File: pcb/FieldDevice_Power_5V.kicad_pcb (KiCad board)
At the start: 2 copper layers, 25 parts, among them J1 Itp_1, J2 V in 6-18V, J3 Itp_2, J4 V out 5V, J5 Vtp_2, J6 Vtp_1, J7 Battery, U1 TPS54232

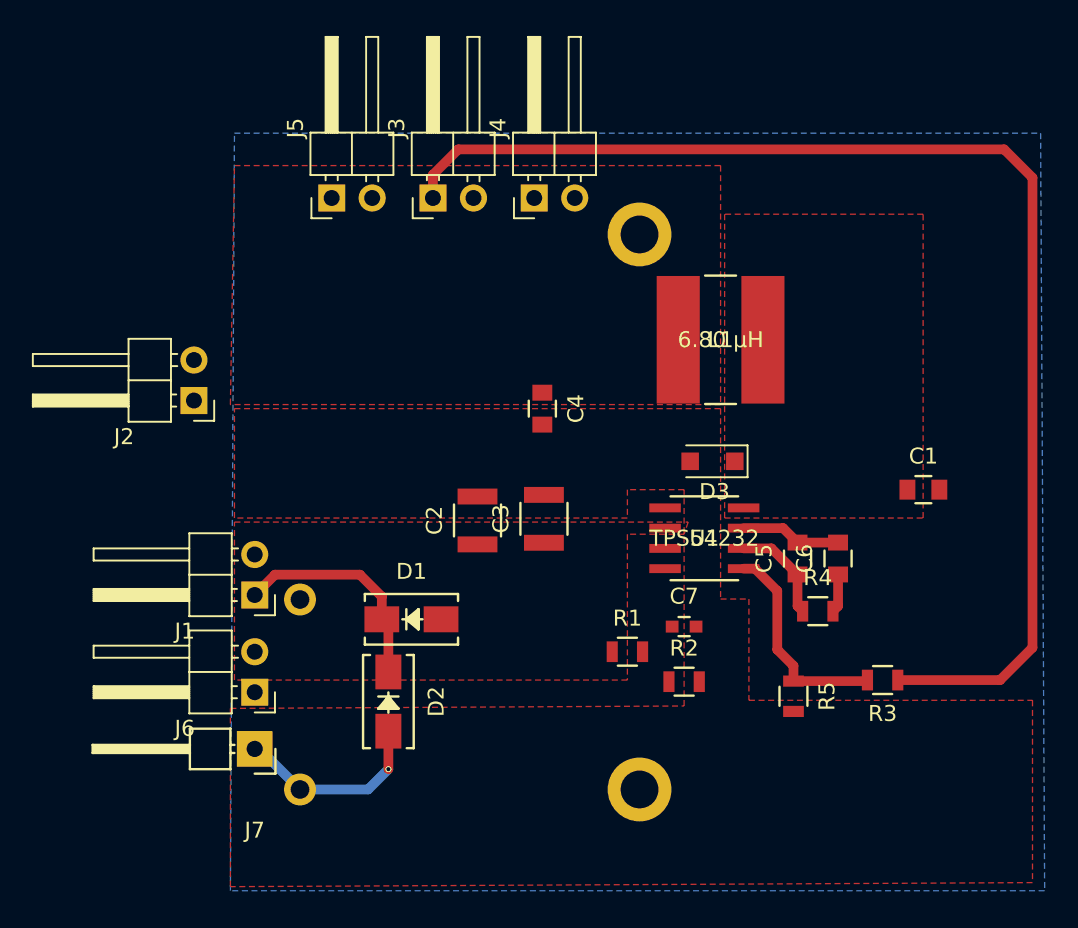
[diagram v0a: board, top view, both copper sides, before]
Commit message: Finishing up the layout
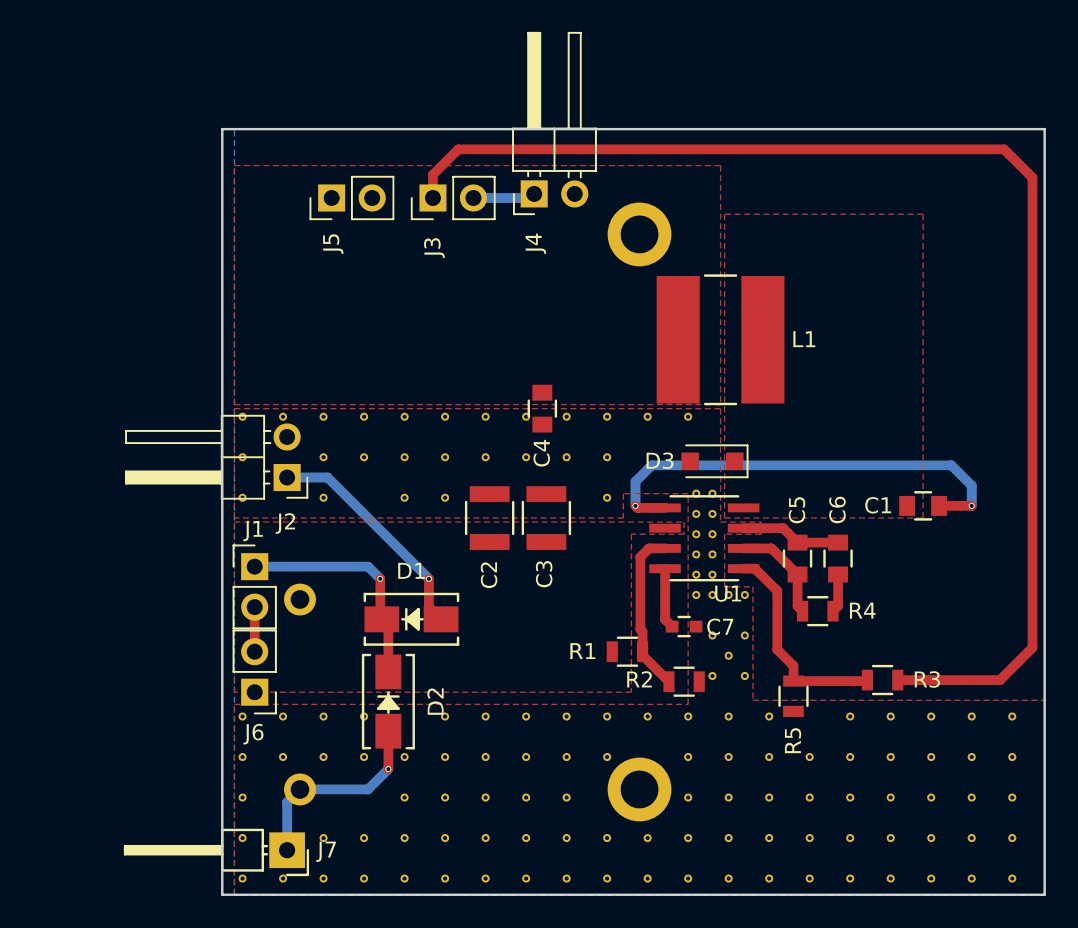
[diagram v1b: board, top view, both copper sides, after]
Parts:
- added ST**: STITCH_VIA, FieldDevice_Power_5V:STITCH_VIA, F.Cu at (95.8, 77.2)
- added ST**: STITCH_VIA, FieldDevice_Power_5V:STITCH_VIA, F.Cu at (94.7, 73.4)
- added ST**: STITCH_VIA, FieldDevice_Power_5V:STITCH_VIA, F.Cu at (93.2, 81.0)
- added ST**: STITCH_VIA, FieldDevice_Power_5V:STITCH_VIA, F.Cu at (90.7, 81.0)
- added ST**: STITCH_VIA, FieldDevice_Power_5V:STITCH_VIA, F.Cu at (88.1, 81.0)
- added ST**: STITCH_VIA, FieldDevice_Power_5V:STITCH_VIA, F.Cu at (85.6, 81.0)
- added ST**: STITCH_VIA, FieldDevice_Power_5V:STITCH_VIA, F.Cu at (83.1, 81.0)
- added ST**: STITCH_VIA, FieldDevice_Power_5V:STITCH_VIA, F.Cu at (80.5, 81.0)
- added ST**: STITCH_VIA, FieldDevice_Power_5V:STITCH_VIA, F.Cu at (78.0, 81.0)
- added ST**: STITCH_VIA, FieldDevice_Power_5V:STITCH_VIA, F.Cu at (72.9, 81.0)
- added ST**: STITCH_VIA, FieldDevice_Power_5V:STITCH_VIA, F.Cu at (70.4, 81.0)
- added ST**: STITCH_VIA, FieldDevice_Power_5V:STITCH_VIA, F.Cu at (67.8, 81.0)
- added ST**: STITCH_VIA, FieldDevice_Power_5V:STITCH_VIA, F.Cu at (94.7, 72.1)
- added ST**: STITCH_VIA, FieldDevice_Power_5V:STITCH_VIA, F.Cu at (65.3, 81.0)
- added ST**: STITCH_VIA, FieldDevice_Power_5V:STITCH_VIA, F.Cu at (88.1, 67.3)
- added ST**: STITCH_VIA, FieldDevice_Power_5V:STITCH_VIA, F.Cu at (78.0, 67.3)
- added ST**: STITCH_VIA, FieldDevice_Power_5V:STITCH_VIA, F.Cu at (75.4, 67.3)
- added ST**: STITCH_VIA, FieldDevice_Power_5V:STITCH_VIA, F.Cu at (70.4, 67.3)
- added ST**: STITCH_VIA, FieldDevice_Power_5V:STITCH_VIA, F.Cu at (65.3, 67.3)
- added ST**: STITCH_VIA, FieldDevice_Power_5V:STITCH_VIA, F.Cu at (88.1, 64.8)
- added ST**: STITCH_VIA, FieldDevice_Power_5V:STITCH_VIA, F.Cu at (85.6, 64.8)
- added ST**: STITCH_VIA, FieldDevice_Power_5V:STITCH_VIA, F.Cu at (83.1, 64.8)
- added ST**: STITCH_VIA, FieldDevice_Power_5V:STITCH_VIA, F.Cu at (80.5, 64.8)
- added ST**: STITCH_VIA, FieldDevice_Power_5V:STITCH_VIA, F.Cu at (94.7, 70.9)
- added ST**: STITCH_VIA, FieldDevice_Power_5V:STITCH_VIA, F.Cu at (78.0, 64.8)
- added ST**: STITCH_VIA, FieldDevice_Power_5V:STITCH_VIA, F.Cu at (75.4, 64.8)
- added ST**: STITCH_VIA, FieldDevice_Power_5V:STITCH_VIA, F.Cu at (72.9, 64.8)
- added ST**: STITCH_VIA, FieldDevice_Power_5V:STITCH_VIA, F.Cu at (70.4, 64.8)
- added ST**: STITCH_VIA, FieldDevice_Power_5V:STITCH_VIA, F.Cu at (65.3, 64.8)
- added ST**: STITCH_VIA, FieldDevice_Power_5V:STITCH_VIA, F.Cu at (93.2, 62.2)
- added ST**: STITCH_VIA, FieldDevice_Power_5V:STITCH_VIA, F.Cu at (90.7, 62.2)
- added ST**: STITCH_VIA, FieldDevice_Power_5V:STITCH_VIA, F.Cu at (88.1, 62.2)
- added ST**: STITCH_VIA, FieldDevice_Power_5V:STITCH_VIA, F.Cu at (85.6, 62.2)
- added ST**: STITCH_VIA, FieldDevice_Power_5V:STITCH_VIA, F.Cu at (83.1, 62.2)
- added ST**: STITCH_VIA, FieldDevice_Power_5V:STITCH_VIA, F.Cu at (94.7, 69.6)
- added ST**: STITCH_VIA, FieldDevice_Power_5V:STITCH_VIA, F.Cu at (80.5, 62.2)
- added ST**: STITCH_VIA, FieldDevice_Power_5V:STITCH_VIA, F.Cu at (78.0, 62.2)
- added ST**: STITCH_VIA, FieldDevice_Power_5V:STITCH_VIA, F.Cu at (75.4, 62.2)
- added ST**: STITCH_VIA, FieldDevice_Power_5V:STITCH_VIA, F.Cu at (72.9, 62.2)
- added ST**: STITCH_VIA, FieldDevice_Power_5V:STITCH_VIA, F.Cu at (70.4, 62.2)
- added ST**: STITCH_VIA, FieldDevice_Power_5V:STITCH_VIA, F.Cu at (67.8, 62.2)
- added ST**: STITCH_VIA, FieldDevice_Power_5V:STITCH_VIA, F.Cu at (65.3, 62.2)
- added ST**: STITCH_VIA, FieldDevice_Power_5V:STITCH_VIA, F.Cu at (93.7, 73.4)
- added ST**: STITCH_VIA, FieldDevice_Power_5V:STITCH_VIA, F.Cu at (93.7, 72.1)
- added ST**: STITCH_VIA, FieldDevice_Power_5V:STITCH_VIA, F.Cu at (93.7, 70.9)
- added ST**: STITCH_VIA, FieldDevice_Power_5V:STITCH_VIA, F.Cu at (93.7, 69.6)
- added ST**: STITCH_VIA, FieldDevice_Power_5V:STITCH_VIA, F.Cu at (94.7, 68.3)
- added ST**: STITCH_VIA, FieldDevice_Power_5V:STITCH_VIA, F.Cu at (93.7, 68.3)
- added ST**: STITCH_VIA, FieldDevice_Power_5V:STITCH_VIA, F.Cu at (94.7, 78.5)
- added ST**: STITCH_VIA, FieldDevice_Power_5V:STITCH_VIA, F.Cu at (113.5, 91.2)
- added ST**: STITCH_VIA, FieldDevice_Power_5V:STITCH_VIA, F.Cu at (111.0, 91.2)
- added ST**: STITCH_VIA, FieldDevice_Power_5V:STITCH_VIA, F.Cu at (108.5, 91.2)
- added ST**: STITCH_VIA, FieldDevice_Power_5V:STITCH_VIA, F.Cu at (105.9, 91.2)
- added ST**: STITCH_VIA, FieldDevice_Power_5V:STITCH_VIA, F.Cu at (103.4, 91.2)
- added ST**: STITCH_VIA, FieldDevice_Power_5V:STITCH_VIA, F.Cu at (100.8, 91.2)
- added ST**: STITCH_VIA, FieldDevice_Power_5V:STITCH_VIA, F.Cu at (98.3, 91.2)
- added ST**: STITCH_VIA, FieldDevice_Power_5V:STITCH_VIA, F.Cu at (95.8, 91.2)
- added ST**: STITCH_VIA, FieldDevice_Power_5V:STITCH_VIA, F.Cu at (93.2, 91.2)
- added ST**: STITCH_VIA, FieldDevice_Power_5V:STITCH_VIA, F.Cu at (90.7, 91.2)
- added ST**: STITCH_VIA, FieldDevice_Power_5V:STITCH_VIA, F.Cu at (96.8, 78.5)
- added ST**: STITCH_VIA, FieldDevice_Power_5V:STITCH_VIA, F.Cu at (88.1, 91.2)
- added ST**: STITCH_VIA, FieldDevice_Power_5V:STITCH_VIA, F.Cu at (85.6, 91.2)
- added ST**: STITCH_VIA, FieldDevice_Power_5V:STITCH_VIA, F.Cu at (83.1, 91.2)
- added ST**: STITCH_VIA, FieldDevice_Power_5V:STITCH_VIA, F.Cu at (80.5, 91.2)
- added ST**: STITCH_VIA, FieldDevice_Power_5V:STITCH_VIA, F.Cu at (78.0, 91.2)
- added ST**: STITCH_VIA, FieldDevice_Power_5V:STITCH_VIA, F.Cu at (75.4, 91.2)
- added ST**: STITCH_VIA, FieldDevice_Power_5V:STITCH_VIA, F.Cu at (72.9, 91.2)
- added ST**: STITCH_VIA, FieldDevice_Power_5V:STITCH_VIA, F.Cu at (70.4, 91.2)
- added ST**: STITCH_VIA, FieldDevice_Power_5V:STITCH_VIA, F.Cu at (67.8, 91.2)
- added ST**: STITCH_VIA, FieldDevice_Power_5V:STITCH_VIA, F.Cu at (65.3, 91.2)
- added ST**: STITCH_VIA, FieldDevice_Power_5V:STITCH_VIA, F.Cu at (96.8, 75.9)
- added ST**: STITCH_VIA, FieldDevice_Power_5V:STITCH_VIA, F.Cu at (113.5, 88.6)
- added ST**: STITCH_VIA, FieldDevice_Power_5V:STITCH_VIA, F.Cu at (111.0, 88.6)
- added ST**: STITCH_VIA, FieldDevice_Power_5V:STITCH_VIA, F.Cu at (108.5, 88.6)
- added ST**: STITCH_VIA, FieldDevice_Power_5V:STITCH_VIA, F.Cu at (105.9, 88.6)
- added ST**: STITCH_VIA, FieldDevice_Power_5V:STITCH_VIA, F.Cu at (103.4, 88.6)
- added ST**: STITCH_VIA, FieldDevice_Power_5V:STITCH_VIA, F.Cu at (100.8, 88.6)
- added ST**: STITCH_VIA, FieldDevice_Power_5V:STITCH_VIA, F.Cu at (98.3, 88.6)
- added ST**: STITCH_VIA, FieldDevice_Power_5V:STITCH_VIA, F.Cu at (95.8, 88.6)
- added ST**: STITCH_VIA, FieldDevice_Power_5V:STITCH_VIA, F.Cu at (93.2, 88.6)
- added ST**: STITCH_VIA, FieldDevice_Power_5V:STITCH_VIA, F.Cu at (90.7, 88.6)
- added ST**: STITCH_VIA, FieldDevice_Power_5V:STITCH_VIA, F.Cu at (94.7, 75.9)
- added ST**: STITCH_VIA, FieldDevice_Power_5V:STITCH_VIA, F.Cu at (88.1, 88.6)
- added ST**: STITCH_VIA, FieldDevice_Power_5V:STITCH_VIA, F.Cu at (85.6, 88.6)
- added ST**: STITCH_VIA, FieldDevice_Power_5V:STITCH_VIA, F.Cu at (83.1, 88.6)
- added ST**: STITCH_VIA, FieldDevice_Power_5V:STITCH_VIA, F.Cu at (80.5, 88.6)
- added ST**: STITCH_VIA, FieldDevice_Power_5V:STITCH_VIA, F.Cu at (78.0, 88.6)
- added ST**: STITCH_VIA, FieldDevice_Power_5V:STITCH_VIA, F.Cu at (75.4, 88.6)
- added ST**: STITCH_VIA, FieldDevice_Power_5V:STITCH_VIA, F.Cu at (72.9, 88.6)
- added ST**: STITCH_VIA, FieldDevice_Power_5V:STITCH_VIA, F.Cu at (70.4, 88.6)
- added ST**: STITCH_VIA, FieldDevice_Power_5V:STITCH_VIA, F.Cu at (65.3, 88.6)
- added ST**: STITCH_VIA, FieldDevice_Power_5V:STITCH_VIA, F.Cu at (113.5, 86.1)
- added ST**: STITCH_VIA, FieldDevice_Power_5V:STITCH_VIA, F.Cu at (94.7, 67.1)
- added ST**: STITCH_VIA, FieldDevice_Power_5V:STITCH_VIA, F.Cu at (111.0, 86.1)
- added ST**: STITCH_VIA, FieldDevice_Power_5V:STITCH_VIA, F.Cu at (108.5, 86.1)
- added ST**: STITCH_VIA, FieldDevice_Power_5V:STITCH_VIA, F.Cu at (105.9, 86.1)
- added ST**: STITCH_VIA, FieldDevice_Power_5V:STITCH_VIA, F.Cu at (103.4, 86.1)
- added ST**: STITCH_VIA, FieldDevice_Power_5V:STITCH_VIA, F.Cu at (100.8, 86.1)
- added ST**: STITCH_VIA, FieldDevice_Power_5V:STITCH_VIA, F.Cu at (98.3, 86.1)
- added ST**: STITCH_VIA, FieldDevice_Power_5V:STITCH_VIA, F.Cu at (95.8, 86.1)
- added ST**: STITCH_VIA, FieldDevice_Power_5V:STITCH_VIA, F.Cu at (93.2, 86.1)
- added ST**: STITCH_VIA, FieldDevice_Power_5V:STITCH_VIA, F.Cu at (85.6, 86.1)
- added ST**: STITCH_VIA, FieldDevice_Power_5V:STITCH_VIA, F.Cu at (83.1, 86.1)
- added ST**: STITCH_VIA, FieldDevice_Power_5V:STITCH_VIA, F.Cu at (93.7, 67.1)
- added ST**: STITCH_VIA, FieldDevice_Power_5V:STITCH_VIA, F.Cu at (80.5, 86.1)
- added ST**: STITCH_VIA, FieldDevice_Power_5V:STITCH_VIA, F.Cu at (78.0, 86.1)
- added ST**: STITCH_VIA, FieldDevice_Power_5V:STITCH_VIA, F.Cu at (75.4, 86.1)
- added ST**: STITCH_VIA, FieldDevice_Power_5V:STITCH_VIA, F.Cu at (65.3, 86.1)
- added ST**: STITCH_VIA, FieldDevice_Power_5V:STITCH_VIA, F.Cu at (113.5, 83.6)
- added ST**: STITCH_VIA, FieldDevice_Power_5V:STITCH_VIA, F.Cu at (111.0, 83.6)
- added ST**: STITCH_VIA, FieldDevice_Power_5V:STITCH_VIA, F.Cu at (108.5, 83.6)
- added ST**: STITCH_VIA, FieldDevice_Power_5V:STITCH_VIA, F.Cu at (105.9, 83.6)
- added ST**: STITCH_VIA, FieldDevice_Power_5V:STITCH_VIA, F.Cu at (103.4, 83.6)
- added ST**: STITCH_VIA, FieldDevice_Power_5V:STITCH_VIA, F.Cu at (100.8, 83.6)
- added ST**: STITCH_VIA, FieldDevice_Power_5V:STITCH_VIA, F.Cu at (96.8, 73.4)
- added ST**: STITCH_VIA, FieldDevice_Power_5V:STITCH_VIA, F.Cu at (98.3, 83.6)
- added ST**: STITCH_VIA, FieldDevice_Power_5V:STITCH_VIA, F.Cu at (95.8, 83.6)
- added ST**: STITCH_VIA, FieldDevice_Power_5V:STITCH_VIA, F.Cu at (93.2, 83.6)
- added ST**: STITCH_VIA, FieldDevice_Power_5V:STITCH_VIA, F.Cu at (88.1, 83.6)
- added ST**: STITCH_VIA, FieldDevice_Power_5V:STITCH_VIA, F.Cu at (85.6, 83.6)
- added ST**: STITCH_VIA, FieldDevice_Power_5V:STITCH_VIA, F.Cu at (83.1, 83.6)
- added ST**: STITCH_VIA, FieldDevice_Power_5V:STITCH_VIA, F.Cu at (80.5, 83.6)
- added ST**: STITCH_VIA, FieldDevice_Power_5V:STITCH_VIA, F.Cu at (78.0, 83.6)
- added ST**: STITCH_VIA, FieldDevice_Power_5V:STITCH_VIA, F.Cu at (75.4, 83.6)
- added ST**: STITCH_VIA, FieldDevice_Power_5V:STITCH_VIA, F.Cu at (72.9, 83.6)
- added ST**: STITCH_VIA, FieldDevice_Power_5V:STITCH_VIA, F.Cu at (95.8, 73.4)
- added ST**: STITCH_VIA, FieldDevice_Power_5V:STITCH_VIA, F.Cu at (70.4, 83.6)
- added ST**: STITCH_VIA, FieldDevice_Power_5V:STITCH_VIA, F.Cu at (67.8, 83.6)
- added ST**: STITCH_VIA, FieldDevice_Power_5V:STITCH_VIA, F.Cu at (65.3, 83.6)
- added ST**: STITCH_VIA, FieldDevice_Power_5V:STITCH_VIA, F.Cu at (113.5, 81.0)
- added ST**: STITCH_VIA, FieldDevice_Power_5V:STITCH_VIA, F.Cu at (111.0, 81.0)
- added ST**: STITCH_VIA, FieldDevice_Power_5V:STITCH_VIA, F.Cu at (108.5, 81.0)
- added ST**: STITCH_VIA, FieldDevice_Power_5V:STITCH_VIA, F.Cu at (105.9, 81.0)
- added ST**: STITCH_VIA, FieldDevice_Power_5V:STITCH_VIA, F.Cu at (103.4, 81.0)
- added ST**: STITCH_VIA, FieldDevice_Power_5V:STITCH_VIA, F.Cu at (98.3, 81.0)
- added ST**: STITCH_VIA, FieldDevice_Power_5V:STITCH_VIA, F.Cu at (95.8, 81.0)
- J1, J3, J5, J6: footprint Pin_Headers:Pin_Header_Angled_1x02_Pitch2.54mm -> Pin_Headers:Pin_Header_Straight_1x02_Pitch2.54mm
- J7: footprint Pin_Headers:Pin_Header_Angled_1x01 -> FieldDevice_Power_5V:Pin_Header_Angled_1x01
- moved J2 7.58 mm to (68.1, 66.0)
- moved J7 6.67 mm to (68.1, 89.4)
- moved J1 1.78 mm to (66.0, 71.6), turned to 0 degrees
- moved C1 1.02 mm to (108.0, 67.8)
- moved C2 0.78 mm to (80.8, 68.6)
- moved J4 0.25 mm to (83.6, 48.3)
- moved C3 0.16 mm to (84.3, 68.6)
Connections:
- net Net-(J3-Pad2) renamed /V5+
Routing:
- net /BOOT: track 0.00 -> 28.8 mm, vias 0 -> 2
- net Net-(D1-Pad2): track 0.00 -> 14.4 mm, vias 0 -> 1
- net /EN: track 0.00 -> 10.6 mm
- net /V5+: track 0.00 -> 3.92 mm
- net /SS: track 0.00 -> 3.82 mm
- net /VIN: track 0.00 -> 2.79 mm
- net /V+: track 14.0 -> 14.2 mm, vias 0 -> 1
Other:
- board outline added: 51.6 x 48 mm
